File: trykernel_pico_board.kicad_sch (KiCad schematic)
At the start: 2 parts, among them J1 Conn_02x20_Odd_Even

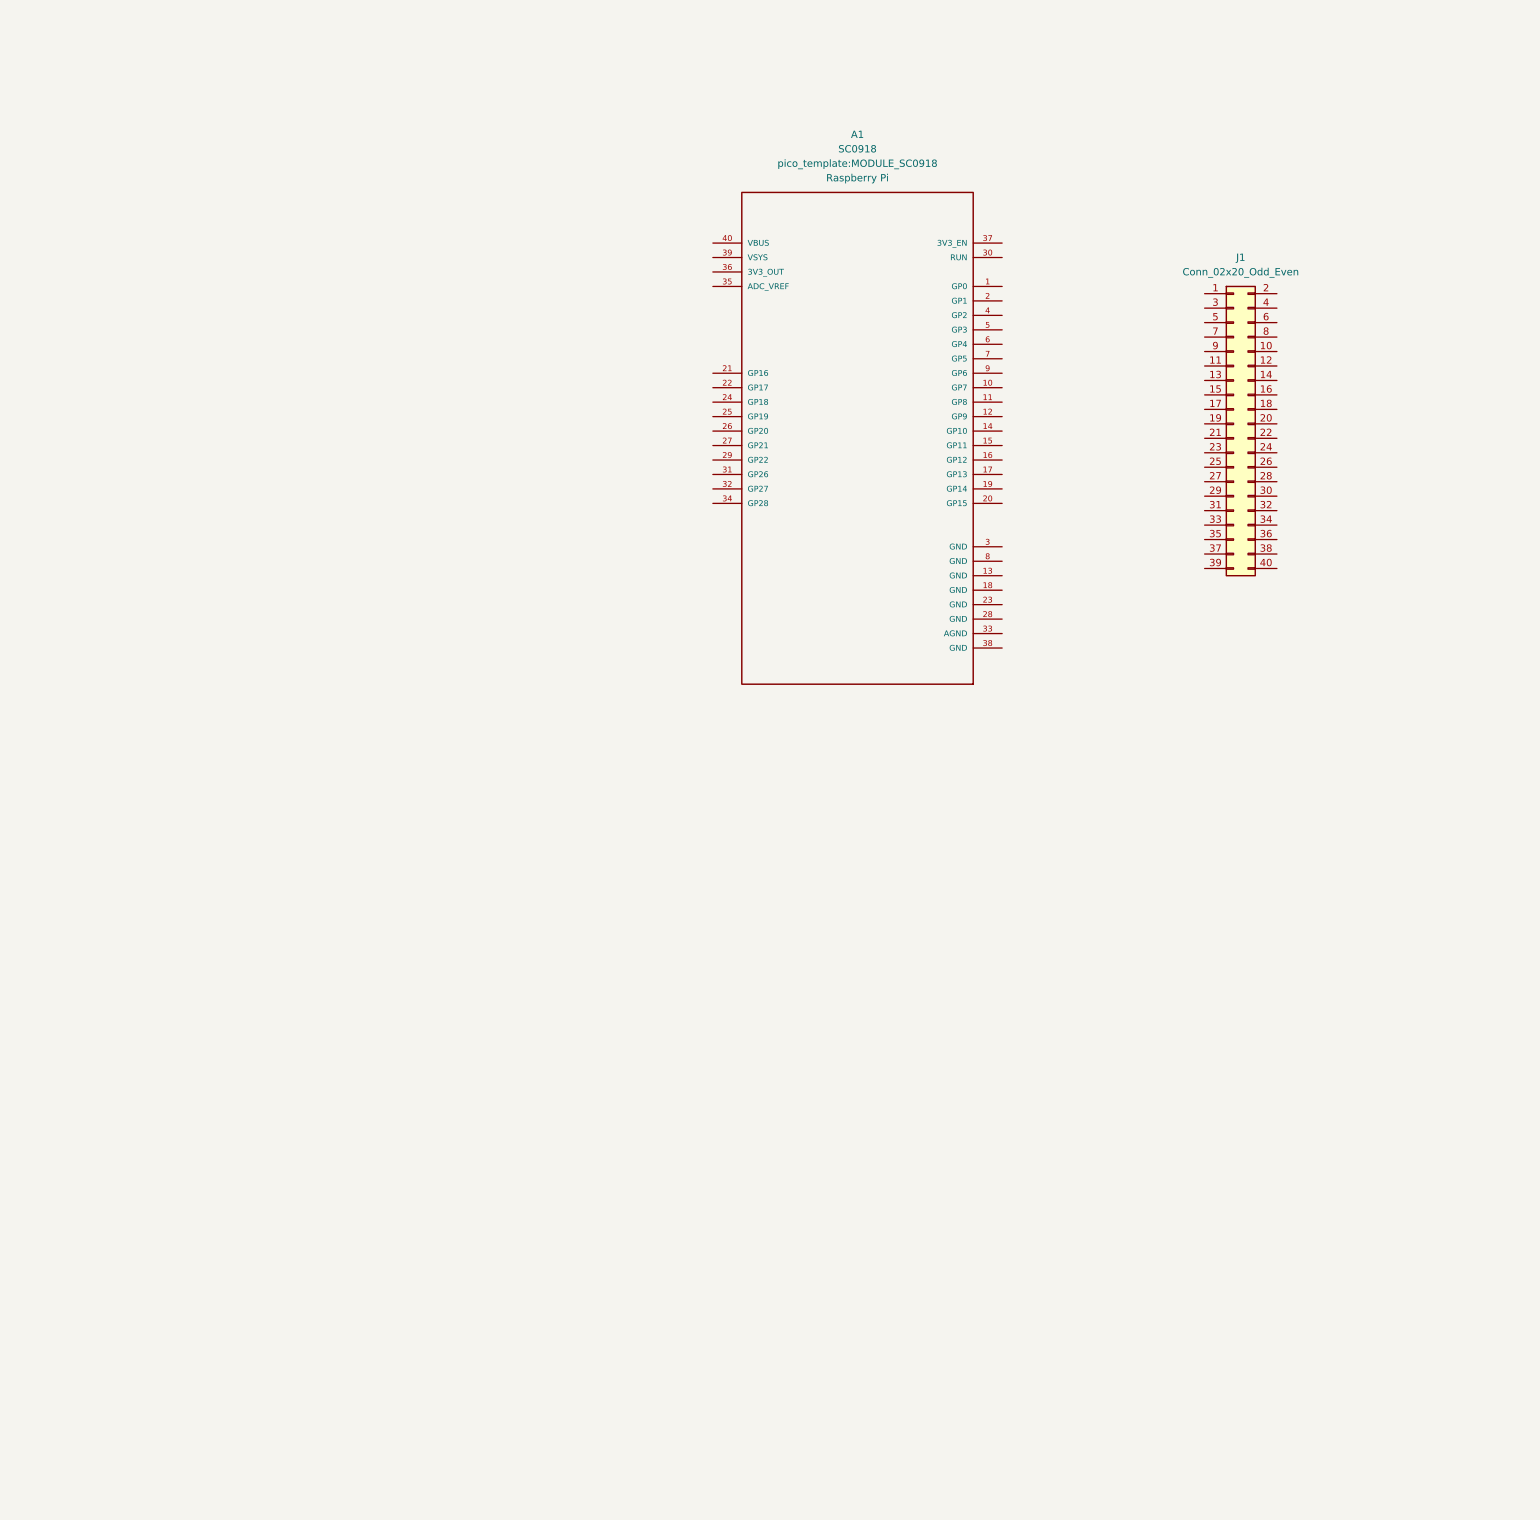
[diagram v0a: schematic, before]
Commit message: version1.0 発注したもの
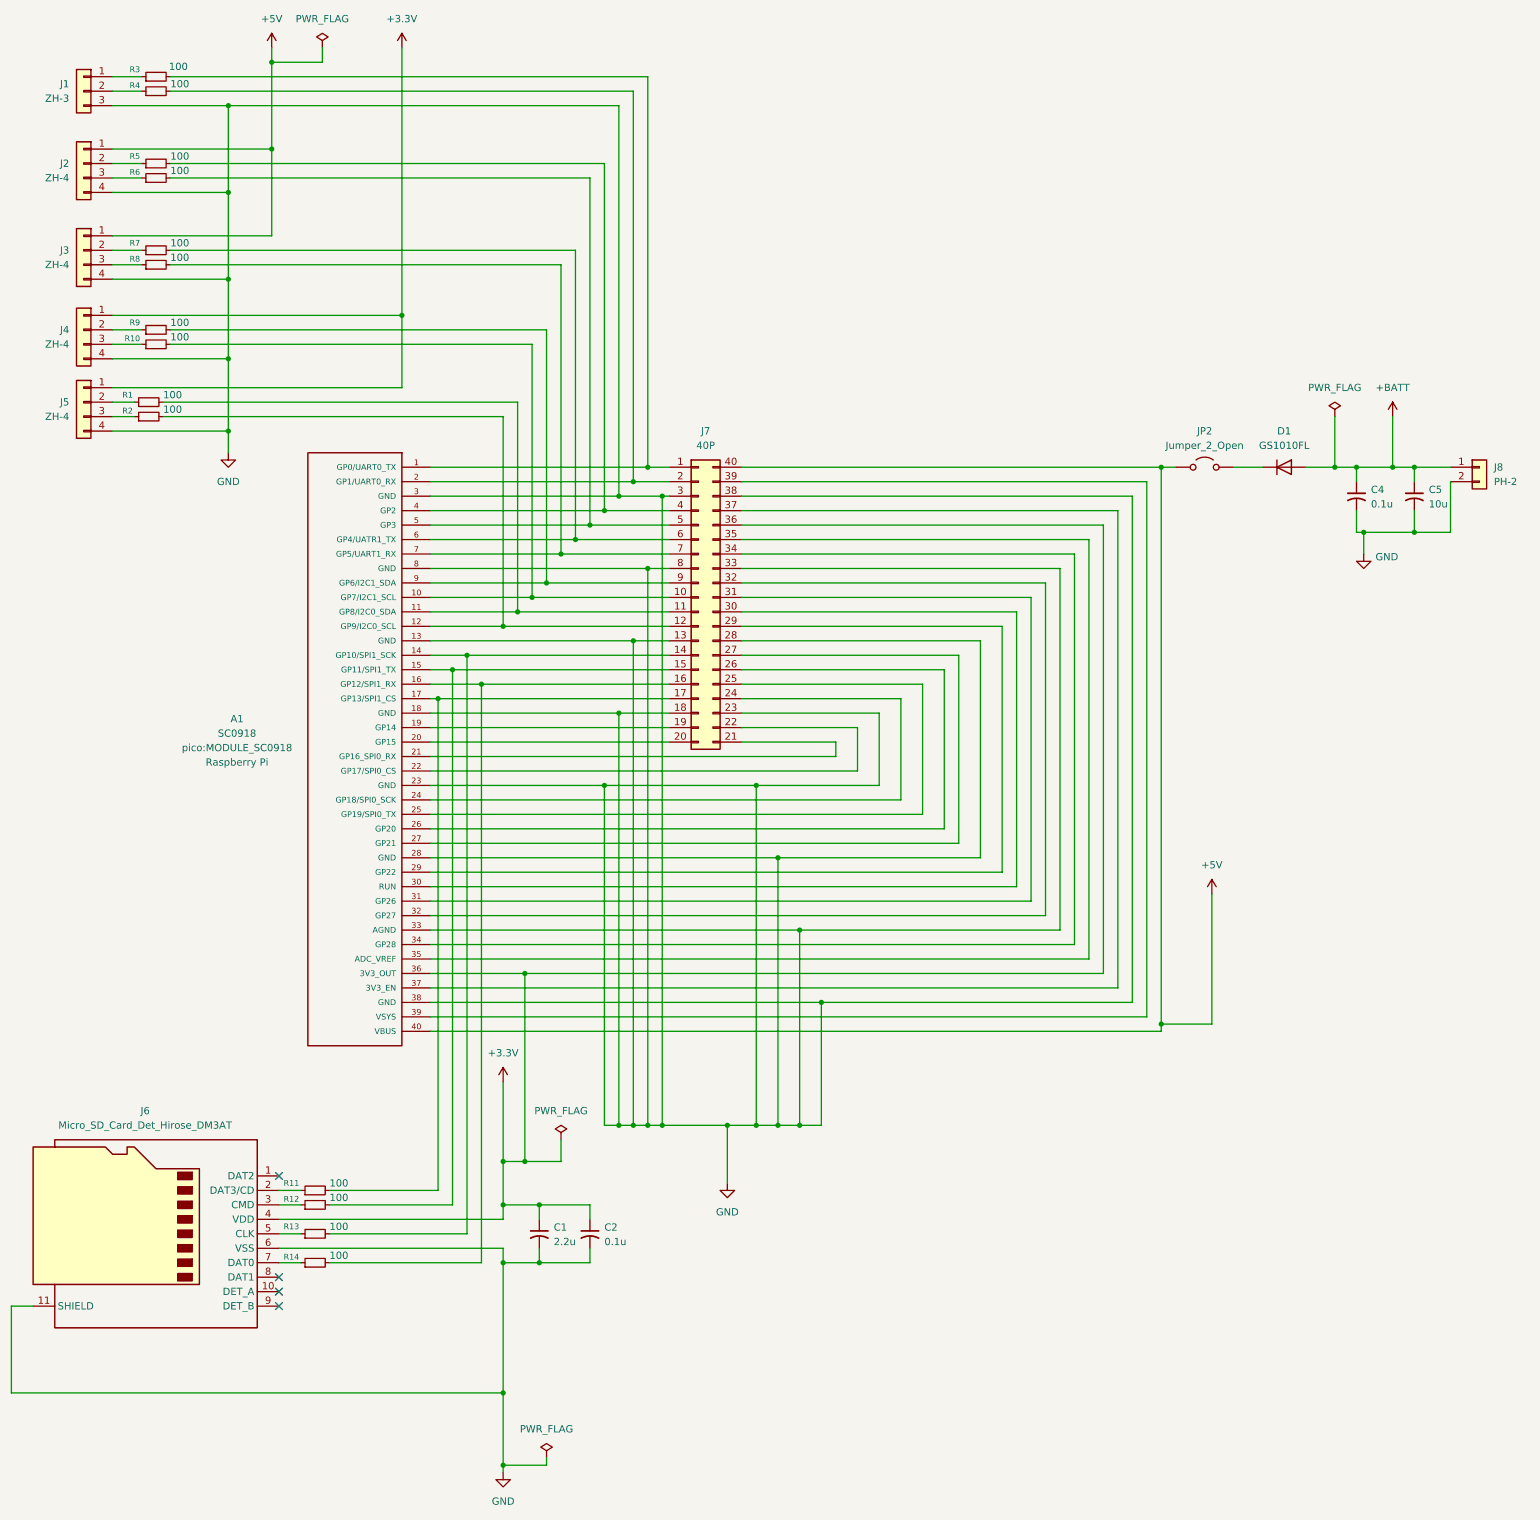
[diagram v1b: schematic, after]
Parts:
- removed J1: Conn_02x20_Odd_Even, RPI_Hat:RPI_Hat_B+, symbol Connector_Generic:Conn_02x20_Odd_Even
- added C1: 2.2u, Capacitor_SMD:C_0603_1608Metric_Pad1.08x0.95mm_HandSolder, symbol Device:C_Small_US
- added C2: 0.1u, Capacitor_SMD:C_0603_1608Metric_Pad1.08x0.95mm_HandSolder, symbol Device:C_Small_US
- added C4: 0.1u, Capacitor_SMD:C_0805_2012Metric_Pad1.18x1.45mm_HandSolder, symbol Device:C_Small_US
- added C5: 10u, Capacitor_SMD:C_0805_2012Metric_Pad1.18x1.45mm_HandSolder, symbol Device:C_Small_US
- added D1: GS1010FL, Diode_SMD:D_SOD-123, symbol Diode:1N4448W
- added J1: ZH-3, Connector_JST:JST_ZH_B3B-ZR_1x03_P1.50mm_Vertical, symbol Connector_Generic:Conn_01x03
- added J2, J3, J4, J5: ZH-4, Connector_JST:JST_ZH_B4B-ZR_1x04_P1.50mm_Vertical, symbol Connector_Generic:Conn_01x04
- added J6: Micro_SD_Card_Det_Hirose_DM3AT, Connector_Card:microSD_HC_Hirose_DM3AT-SF-PEJM5, symbol Connector:Micro_SD_Card_Det_Hirose_DM3AT
- added J7: 40P, RPI_Hat:RPI_Hat_B+, symbol Connector_Generic:Conn_02x20_Counter_Clockwise
- added J8: PH-2, Connector_JST:JST_PH_B2B-PH-K_1x02_P2.00mm_Vertical, symbol Connector_Generic:Conn_01x02
- added JP2: Jumper_2_Open, module:Pin_Header_Straight_1x02, symbol Jumper:Jumper_2_Open
- added R1, R10, R11, R12, R13, R14, R2, R3, R4, R5, R6, R7, R8, R9: 100, Resistor_SMD:R_0603_1608Metric_Pad0.98x0.95mm_HandSolder, symbol Device:R_Small
- A1: footprint pico_template:MODULE_SC0918 -> pico:MODULE_SC0918
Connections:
- net at A1.1 (GP0/UART0_TX): now also J7.1 (Pin_1), R3.2
- net at A1.10 (GP7/I2C1_SCL): now also J7.10 (Pin_10), R10.2
- net at A1.11 (GP8/I2C0_SDA): now also J7.11 (Pin_11), R1.2
- net at A1.12 (GP9/I2C0_SCL): now also J7.12 (Pin_12), R2.2
- net GND: now reaches A1.13 (GND)
- net GND: now also A1.18 (GND), A1.23 (GND), A1.28 (GND), A1.3 (GND), A1.33 (AGND), A1.38 (GND), A1.8 (GND), C1.2, C2.2, C4.2, C5.2, J1.3 (Pin_3), J2.4 (Pin_4), J3.4 (Pin_4), J4.4 (Pin_4), J5.4 (Pin_4), J6.11 (SHIELD), J6.6 (VSS), J7.13 (Pin_13), J7.18 (Pin_18), J7.23 (Pin_23), J7.28 (Pin_28), J7.3 (Pin_3), J7.33 (Pin_33), J7.38 (Pin_38), J7.8 (Pin_8), J8.2 (Pin_2)
- net at A1.14 (GP10/SPI1_SCK): now also J7.14 (Pin_14), R13.2
- net at A1.15 (GP11/SPI1_TX): now also J7.15 (Pin_15), R12.2
- net at A1.16 (GP12/SPI1_RX): now also J7.16 (Pin_16), R14.2
- net at A1.17 (GP13/SPI1_CS): now also J7.17 (Pin_17), R11.2
- net at A1.19 (GP14): now also J7.19 (Pin_19)
- net at A1.2 (GP1/UART0_RX): now also J7.2 (Pin_2), R4.2
- net at A1.20 (GP15): now also J7.20 (Pin_20)
- net at A1.21 (GP16_SPI0_RX): now also J7.21 (Pin_21)
- net at A1.22 (GP17/SPI0_CS): now also J7.22 (Pin_22)
- net at A1.24 (GP18/SPI0_SCK): now also J7.24 (Pin_24)
- net at A1.25 (GP19/SPI0_TX): now also J7.25 (Pin_25)
- net at A1.26 (GP20): now also J7.26 (Pin_26)
- net at A1.27 (GP21): now also J7.27 (Pin_27)
- net at A1.29 (GP22): now also J7.29 (Pin_29)
- net at A1.30 (RUN): now also J7.30 (Pin_30)
- net at A1.31 (GP26): now also J7.31 (Pin_31)
- net at A1.32 (GP27): now also J7.32 (Pin_32)
- net at A1.34 (GP28): now also J7.34 (Pin_34)
- net at A1.35 (ADC_VREF): now also J7.35 (Pin_35)
- net +3.3V: now reaches A1.36 (3V3_OUT)
- net +3.3V: now also C1.1, C2.1, J4.1 (Pin_1), J5.1 (Pin_1), J6.4 (VDD), J7.36 (Pin_36)
- net at A1.37 (3V3_EN): now also J7.37 (Pin_37)
- net at A1.39 (VSYS): now also J7.39 (Pin_39)
- net at A1.4 (GP2): now also J7.4 (Pin_4), R5.2
- net +5V: now reaches A1.40 (VBUS)
- net +5V: now also J2.1 (Pin_1), J3.1 (Pin_1), J7.40 (Pin_40), JP2.1 (A)
- net at A1.5 (GP3): now also J7.5 (Pin_5), R6.2
- net at A1.6 (GP4/UATR1_TX): now also J7.6 (Pin_6), R7.2
- net at A1.7 (GP5/UART1_RX): now also J7.7 (Pin_7), R8.2
- net at A1.9 (GP6/I2C1_SDA): now also J7.9 (Pin_9), R9.2
- new net: J6.2 (DAT3/CD), R11.1
- new net: J4.3 (Pin_3), R10.1
- new net: J3.3 (Pin_3), R8.1
- new net: J5.2 (Pin_2), R1.1
- new net: J3.2 (Pin_2), R7.1
- new net: D1.1 (K), JP2.2 (B)
- new net: J4.2 (Pin_2), R9.1
- new net: J6.3 (CMD), R12.1
- new net: J6.5 (CLK), R13.1
- new net: J6.7 (DAT0), R14.1
- new net: J5.3 (Pin_3), R2.1
- new net: J1.1 (Pin_1), R3.1
- new net: J2.2 (Pin_2), R5.1
- new net: J2.3 (Pin_3), R6.1
- new net: J1.2 (Pin_2), R4.1
- new net +BATT: C4.1, C5.1, D1.2 (A), J8.1 (Pin_1)
- no-connect marks 0 -> 4
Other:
- moved on the sheet: A1
